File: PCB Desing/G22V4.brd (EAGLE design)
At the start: 120.3 x 45.7 mm, 20 parts, among them X2 5566-4

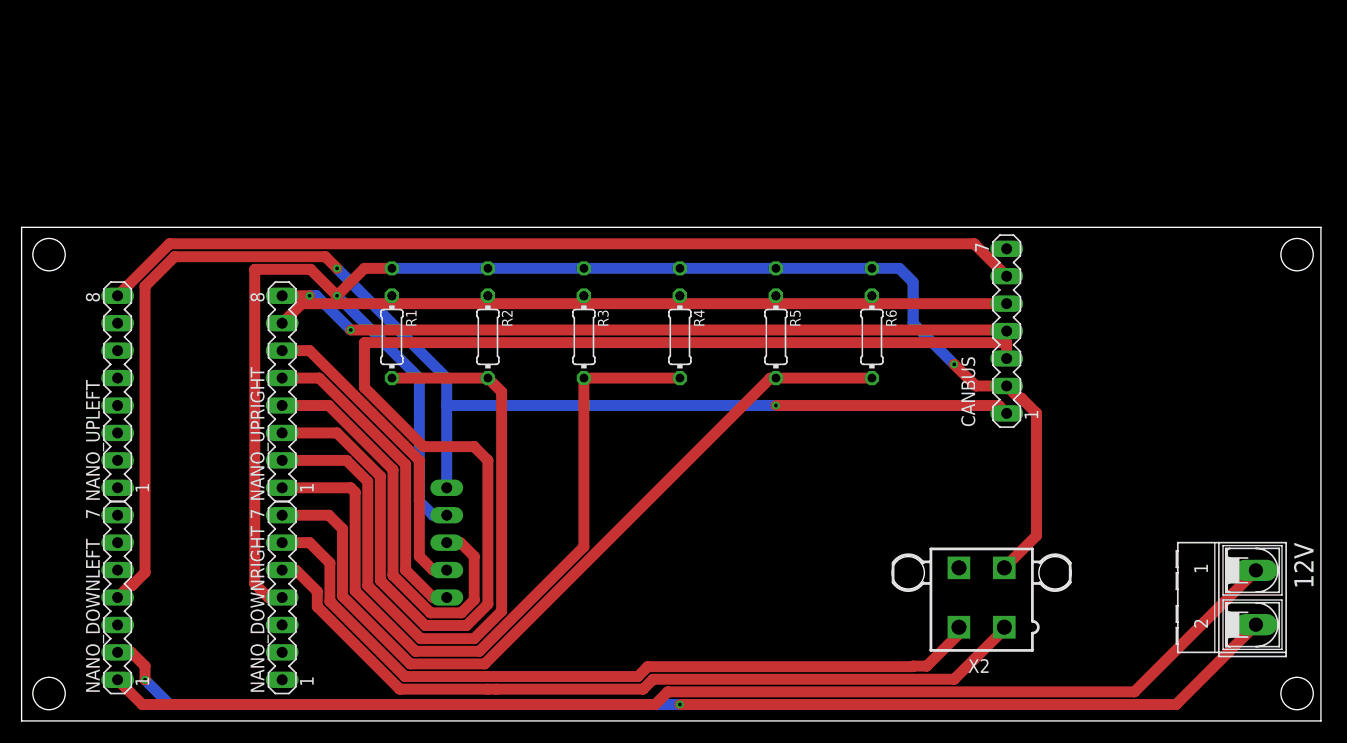
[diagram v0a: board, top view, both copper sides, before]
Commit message: V4 donete
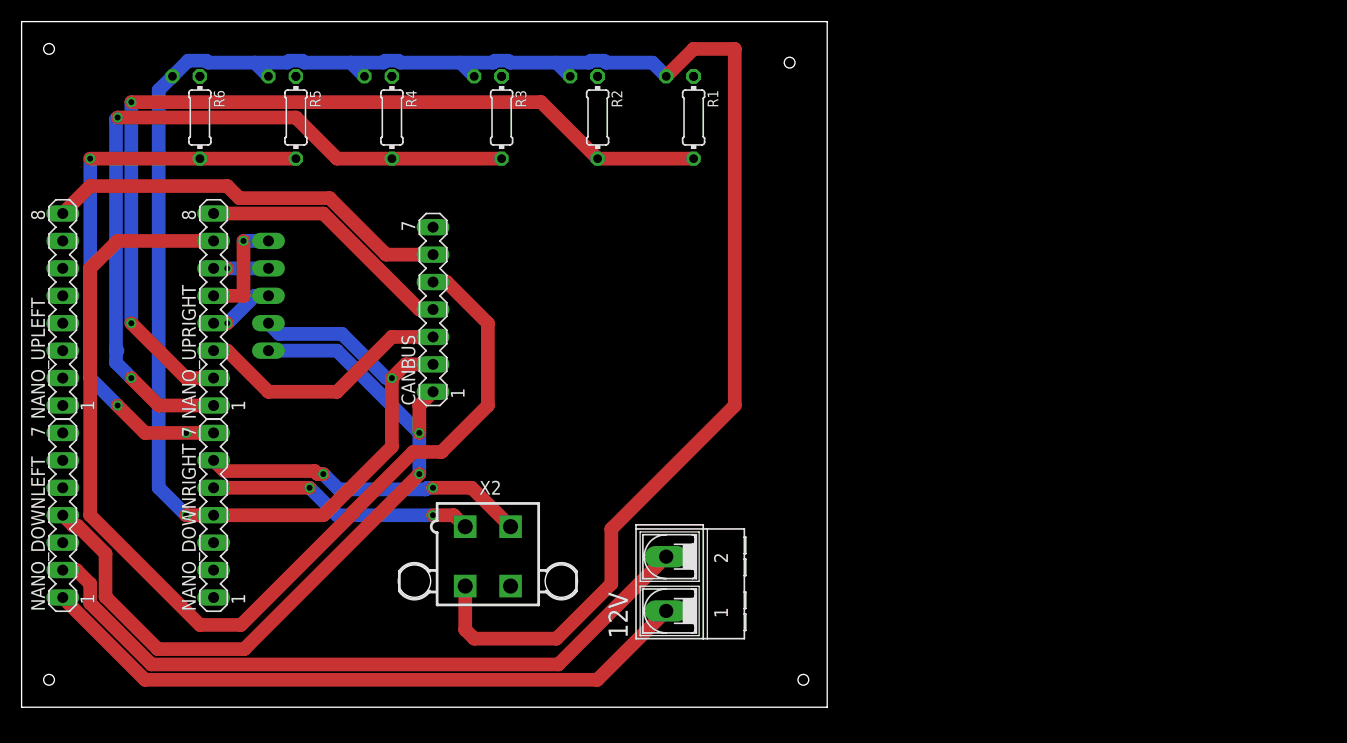
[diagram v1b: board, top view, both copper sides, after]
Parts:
- moved RPM6 66.3 mm to (15.2, 58.4), turned to 0 degrees
- moved R6 65.5 mm to (16.5, 54.6)
- moved 12V 54.6 mm to (59.7, 11.4), turned to 90 degrees
- moved CANBUS 53.2 mm to (38.1, 36.8)
- moved RPM5 49.5 mm to (24.1, 58.4), turned to 0 degrees
- moved R5 48.9 mm to (25.4, 54.6)
- moved X2 45.9 mm to (43.2, 14.0), turned to 180 degrees
- moved R1 34.5 mm to (62.2, 54.6)
- moved RPM4 33.8 mm to (33.0, 58.4), turned to 0 degrees
- moved R4 33.5 mm to (34.3, 54.6)
- moved RPM1 32.8 mm to (61.0, 58.4), turned to 0 degrees
- moved MATRIX 28.2 mm to (22.9, 38.1), turned to 270 degrees
- moved R2 22.7 mm to (53.3, 54.6)
- moved R3 21.7 mm to (44.5, 54.6)
- moved RPM2 21.0 mm to (52.1, 58.4), turned to 0 degrees
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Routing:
- net CS_CAN: track 125.6 -> 24.0 mm
- net VCC: track 126.1 -> 72.5 mm
- net D2: track 74.7 -> 24.8 mm, vias 0 -> 2
- net VIN: track 111.5 -> 61.7 mm
- net SCK: track 85.6 -> 38.0 mm
- net MISO: track 68.5 -> 24.0 mm, vias 2 -> 0
- net D3: track 72.1 -> 30.2 mm, vias 0 -> 2
- net DIN: track 39.1 -> 6.13 mm, vias 0 -> 1
- net MOSI: track 67.8 -> 99.1 mm
- net CS_MATRIX: track 28.9 -> 5.08 mm, vias 0 -> 1
- net GND: track 266.5 -> 289.2 mm, vias 4 -> 3
- net D4: track 74.9 -> 52.9 mm, vias 0 -> 6
- net CLK: track 30.7 -> 10.2 mm, vias 0 -> 1
- net D6: track 66.1 -> 84.4 mm, vias 0 -> 2
- net D5: track 68.1 -> 70.8 mm, vias 0 -> 2
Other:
- board size 120.3 x 45.7 mm -> 74.6 x 63.5 mm
